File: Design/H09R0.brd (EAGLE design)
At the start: 34.6 x 30 mm, 32 parts, among them P2 HEXABIT_17.32_NO_P6, P3 691311500102, U2 AD8495ARMZ-R7, U3 TLVH431ACDBVR, X1 XTALL_CSTCE8M00G52

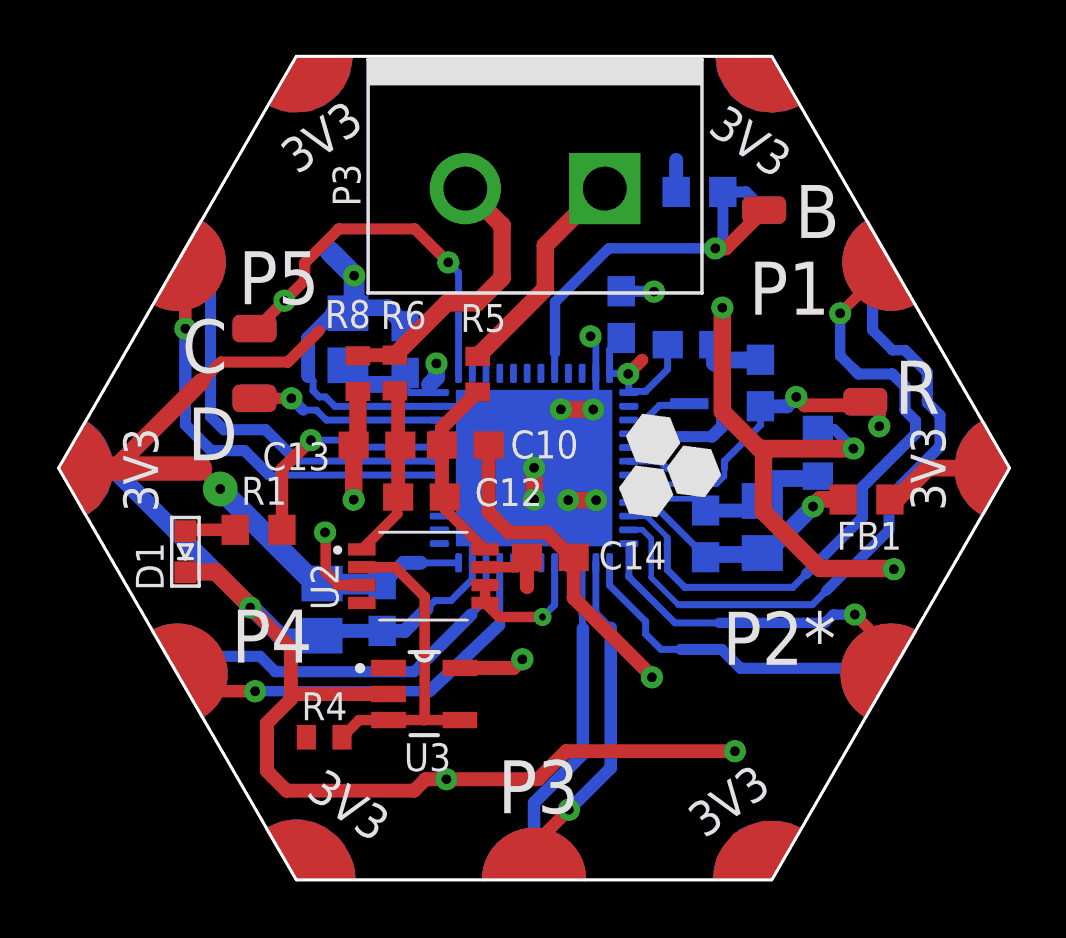
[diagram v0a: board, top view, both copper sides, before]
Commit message: - Deleted old output files - Changed MCU to G0 - New schematic - New layout - Generated documentation - Generated BOM
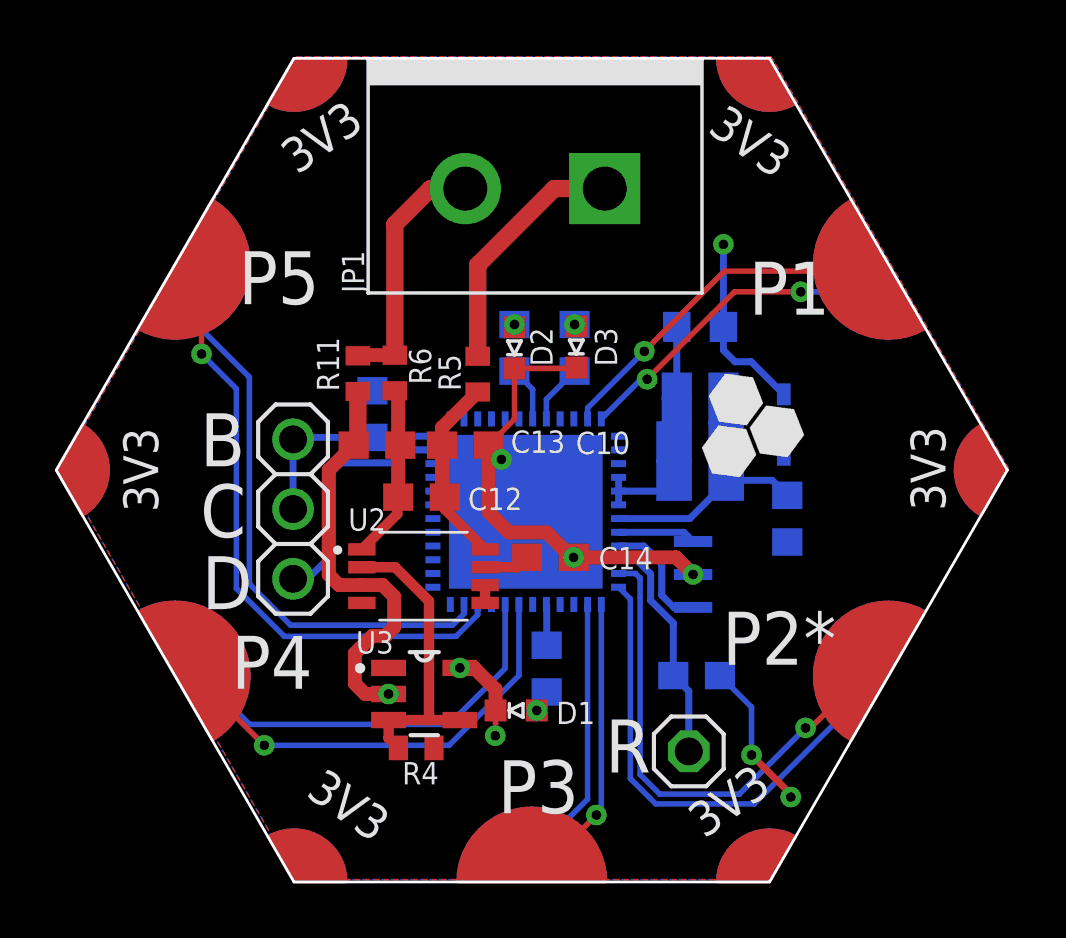
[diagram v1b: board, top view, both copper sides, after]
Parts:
- removed B, C, D: PAD1, Hexabitz:PAD1
- removed C3, C4: 4.7uF, Hexabitz:C-0805-POL
- removed C5: 10nF, Hexabitz:C-0603
- removed C6: 100nF, Hexabitz:C-0603
- removed U1: (no value), Hexabitz:STM32F091CBU6
- added D2: ORANGE, HEXABITZ_USER_INTERFACE_PARTS:VLMS1300-GS08
- added D3: YELLOW, HEXABITZ_USER_INTERFACE_PARTS:VLMS1300-GS08
- added D5: BOURNS_CDSOD323-T03SCBOURNS_CDSOD323-T03SC_0_0, HEXABITZ_RCLS:BOURNS_CDSOD323-T03SC_0
- added R11: 1M, Hexabitz:R-0402
- added R9: 270.0R, HEXABITZ_RCLS:R-0603
- added SWD1: (no value), pinhead:1X03
- added U4: STM32G0B1CEU6QFN_B1CEU6_STM-L, HEXABITZ_ICs:QFN_B1CEU6_STM-L
- C1: value 100nF -> 1uF; device Hexabitz:C-0603 -> HEXABITZ_RCLS:C-0805
- C2: value 1.00uF -> 100nF; device Hexabitz:C-0805-POL -> HEXABITZ_RCLS:C-0603
- C7, C8: device Hexabitz:C-0603 -> HEXABITZ_RCLS:C-0603
- C9: value 100nF -> 4.7uF; device Hexabitz:C-0603 -> HEXABITZ_RCLS:C-0805
- D1: value VLMS1300-GS08 -> RED; device Hexabitz:VLMS1300-GS08 -> HEXABITZ_USER_INTERFACE_PARTS:VLMS1300-GS08
- FB1: device Hexabitz:FB-TDK_MMZ1608Y300B -> HEXABITZ_RCLS:FB-0603
- P2: device Hexabitz:HEXABIT_17.32_NO_P6 -> hexabitz_connectors:HEXABIT_17.32_NO_P6
- R: value PAD1 -> R; device Hexabitz:PAD1 -> HEXABITZ_USER_INTERFACE_PARTS:1X01
- R1: value 270.0R -> 0.0R; device Hexabitz:R-0603 -> HEXABITZ_RCLS:R-0603
- R2: value 10.0K -> 270R; device Hexabitz:R-0603 -> HEXABITZ_RCLS:R-0603
- R3: value 0.0R -> 10K; device Hexabitz:R-0603 -> HEXABITZ_RCLS:R-0603
- R8: value 1M -> 270.0R; device Hexabitz:R-0402 -> HEXABITZ_RCLS:R-0603
- X1: device Hexabitz:XTALL_CSTCE8M00G52 -> HEXABITZ_RCLS:XTALL_CSTCE8M00G52
- moved R1 19.3 mm to (26.5, 13.2), flipped to the bottom, turned to 90 degrees
- moved R2 18.2 mm to (17.8, 7.70), turned to 270 degrees
- moved R3 16.3 mm to (11.4, 17.0)
- moved R 14.3 mm to (23.0, 4.68)
- moved C7 13.6 mm to (23.4, 17.1), turned to 180 degrees
- moved D1 13.4 mm to (16.7, 6.17), turned to 270 degrees
- moved FB1 8.73 mm to (23.4, 20.1), flipped to the bottom, turned to 180 degrees
- moved R8 7.95 mm to (18.8, 19.4), flipped to the bottom, turned to 270 degrees
- moved C2 5.92 mm to (23.2, 7.44), turned to 180 degrees
- moved X1 5.02 mm to (23.1, 11.1), turned to 180 degrees
- moved C9 4.95 mm to (23.4, 14.6)
- moved C8 3.88 mm to (23.4, 18.0), turned to 180 degrees
- moved R4 3.37 mm to (13.0, 4.80), turned to 0 degrees
- moved C1 3.07 mm to (23.4, 16.0), turned to 180 degrees
- moved P2 0.11 mm to (17.2, 14.9)
- renumbered P3 to JP1
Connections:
- removed net B: B.P$1, B.P$2, R2.2, U1.P$44
- removed net N$1: D.P$1, D.P$2, U1.P$34
- removed net N$2: C.P$1, C.P$2, U1.P$37
- removed net R: C1.1, R.P$1, R.P$2, U1.P$7
- removed net USART1_RX: P2.23, U1.P$31
- removed net USART1_TX: P2.17, U1.P$30
- new net CLK: R3.2, SWD1.1, SWD1.2, U4.36
- new net DATA: SWD1.3, U4.35
- new net N$16: D1.A, R2.2
- new net N$17: R8.2, U4.44
- new net N$18: R9.2, U4.43
- new net N$19: D2.A, R9.1
- new net N$20: D3.A, R8.1
- new net USART5_RX: P2.PAD_PD4, U4.20
- new net USART5_TX: P2.PAD_PU4, U4.19
- net GND: now also C2.2, D2.C, D3.C, D5.1, P2.PAD_PD10, P2.PAD_PD11, P2.PAD_PD12, P2.PAD_PD7, P2.PAD_PD8, P2.PAD_PD9, R1.1, R11.1, U4.49; no longer C1.2, C3.2, C4.2, C6.2, C7.2, C8.2, C9.2, P2.10, P2.11, P2.12, P2.7, P2.8, P2.9, R2.1, R8.1, U1.EP, U1.P$23, U1.P$35, U1.P$47
- net N$10: now also U4.8, X1.P$3; no longer D1.A, R1.1
- net N$14: now also C2.1, R.1, U4.10; no longer U1.P$5, X1.P$1
- net N$15: now also R2.1, U4.17; no longer U1.P$6, X1.P$3
- net N$8: now also U4.9, X1.P$1; no longer R1.2, U1.P$32
- net TEMP1: no longer U1.P$17
- net TYPE_K_THC_IN-: now also R11.2; no longer R8.2
- net USART2_RX: now also P2.PAD_PD3, U4.14; no longer P2.20, U1.P$13
- net USART2_TX: now also P2.PAD_PU3, U4.13; no longer P2.14, U1.P$12
- net USART3_RX: now also P2.PAD_PD5, U4.23; no longer P2.22, U1.P$22
- net USART3_TX: now also P2.PAD_PU5, U4.22; no longer P2.16, U1.P$21
- net USART4_RX: now also P2.PAD_PD2, U4.12; no longer P2.19, U1.P$11
- net USART4_TX: now also P2.PAD_PU2, U4.11; no longer P2.13, U1.P$10
- net USART6_RX: now also P2.PAD_PD1, U4.48; no longer P2.21, U1.P$15
- net USART6_TX: now also P2.PAD_PU1, U4.47; no longer P2.15, U1.P$14
- net VDD: now also D5.2, P2.PAD_PU10, P2.PAD_PU11, P2.PAD_PU12, P2.PAD_PU7, P2.PAD_PU8, P2.PAD_PU9; no longer C3.1, C4.1, C6.1, C7.1, C8.1, C9.1, P2.1, P2.2, P2.3, P2.4, P2.5, P2.6, U1.P$1, U1.P$24, U1.P$36, U1.P$48
- net VDDA: now also C1.1, C7.1, C8.1, C9.1, U4.4, U4.5, U4.6; no longer C2.1, C5.1, U1.P$9
- net VSSA: now also C1.2, C7.2, C8.2, C9.2, R1.2, U4.7; no longer C2.2, C5.2, R3.2, U1.P$8
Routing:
- net GND: track 150.9 -> 40.3 mm, vias 19 -> 8
- net VDD: track 45.4 -> 8.40 mm, vias 3 -> 1
- net USART5_TX: track 0.00 -> 17.4 mm, vias 0 -> 1
- net USART1_TX: track 16.2 -> 0.00 mm, vias 1 -> 0
- net B: track 15.6 -> 0.00 mm, vias 1 -> 0
- net USART5_RX: track 0.00 -> 15.5 mm
- net N$2: track 15.2 -> 0.00 mm, vias 2 -> 0
- net USART1_RX: track 14.7 -> 0.00 mm
- net R: track 13.7 -> 0.00 mm, vias 2 -> 0
- net DATA: track 0.00 -> 8.81 mm
- net N$1: track 8.41 -> 0.00 mm, vias 1 -> 0
- net USART3_RX: track 13.5 -> 21.7 mm
- net CLK: track 0.00 -> 7.69 mm
- net USART3_TX: track 15.6 -> 22.3 mm
- net USART4_RX: track 24.0 -> 18.8 mm
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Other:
- board text added: "H09R01"
- board text removed: "H09R00"
- board text removed: "R"
- board text removed: "Total Thickness 1.6 mm --------------------------------------------------------- copper_top.gbr : Top Conductor - Copper: Thickness 0.035 mm Dielectric - FR-4: copper_bottom.gbr : Bottom Conductor - Copper: Thickness 0.035 mm"
